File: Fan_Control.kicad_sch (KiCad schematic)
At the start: 7 parts, among them IC1 ADT7470ARQZ-REEL7

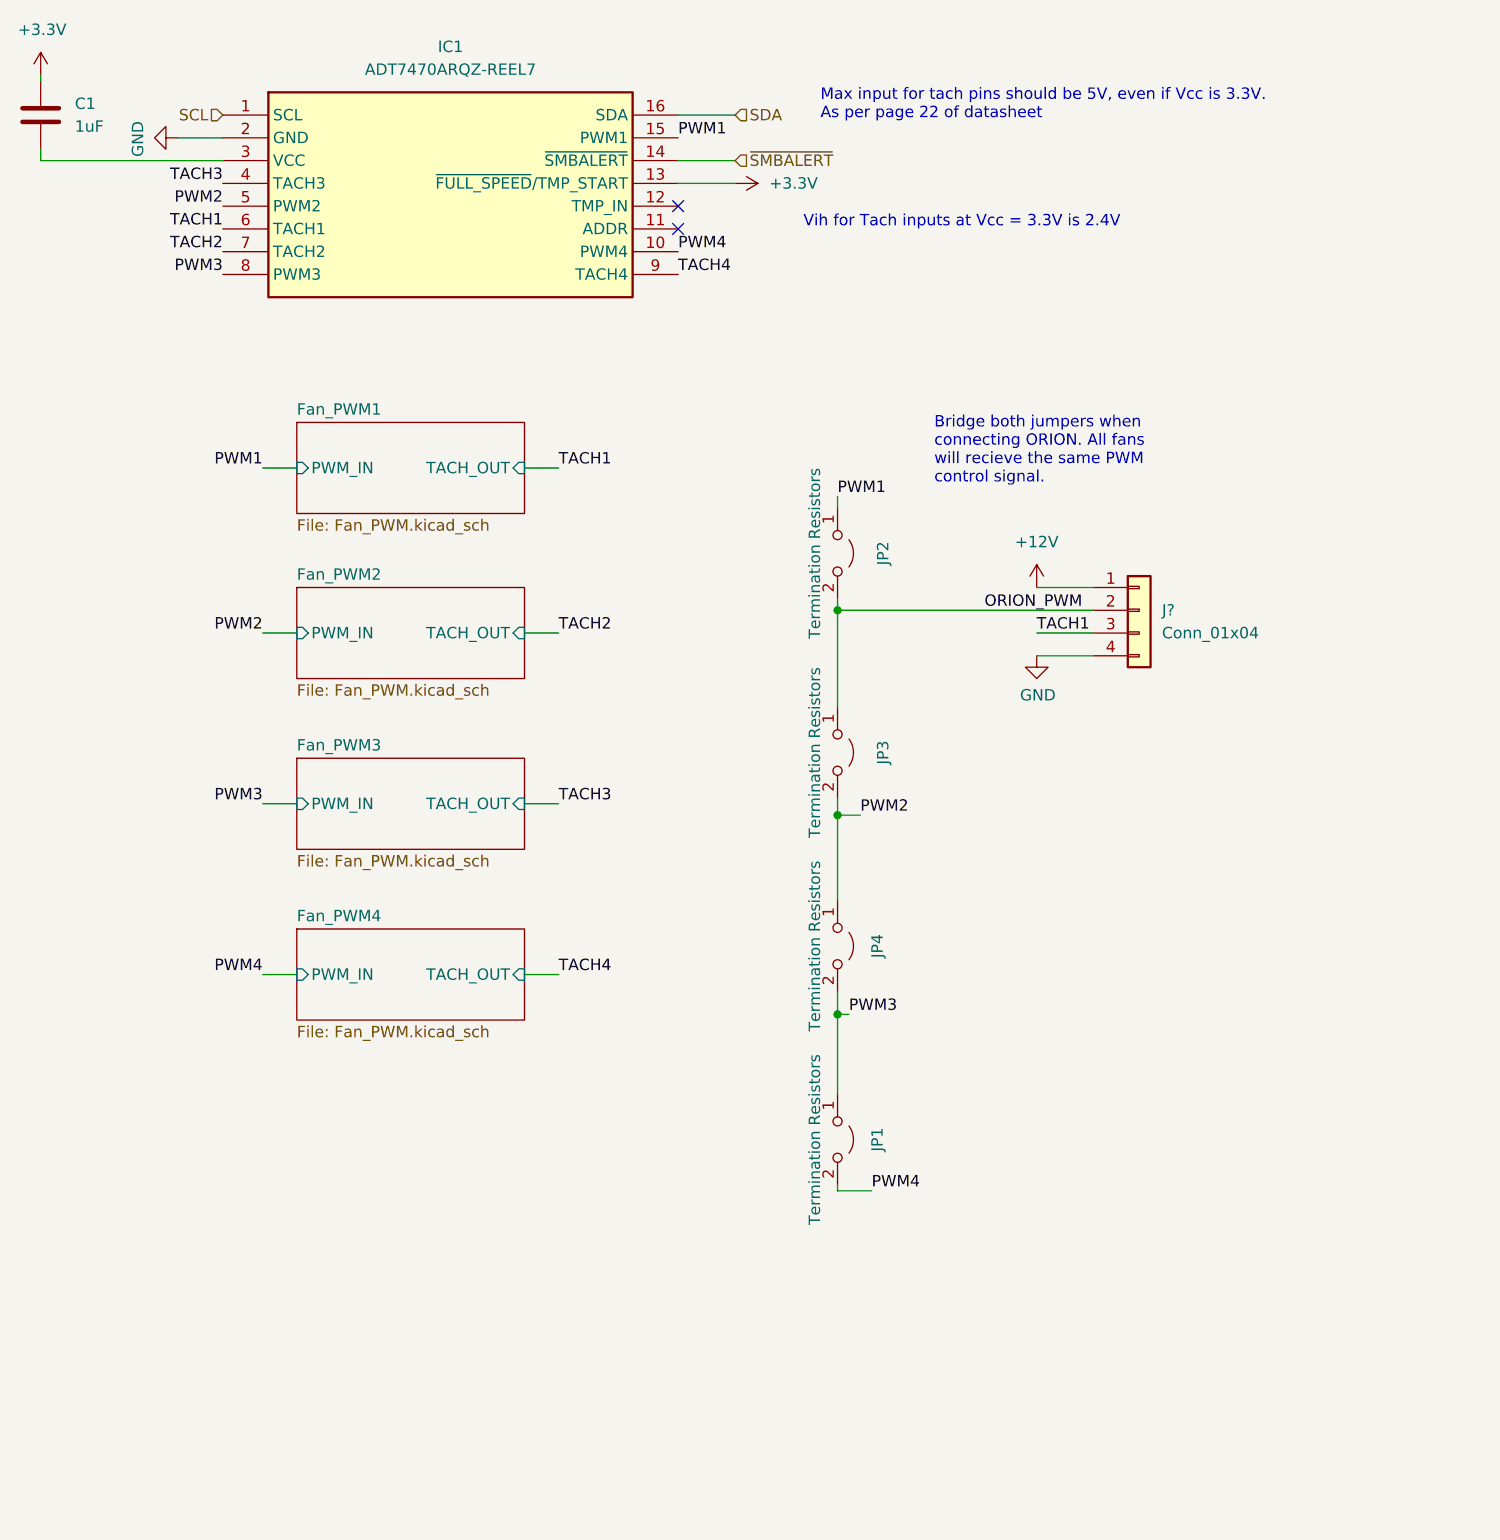
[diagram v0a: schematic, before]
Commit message: why your schematic so broken >:(
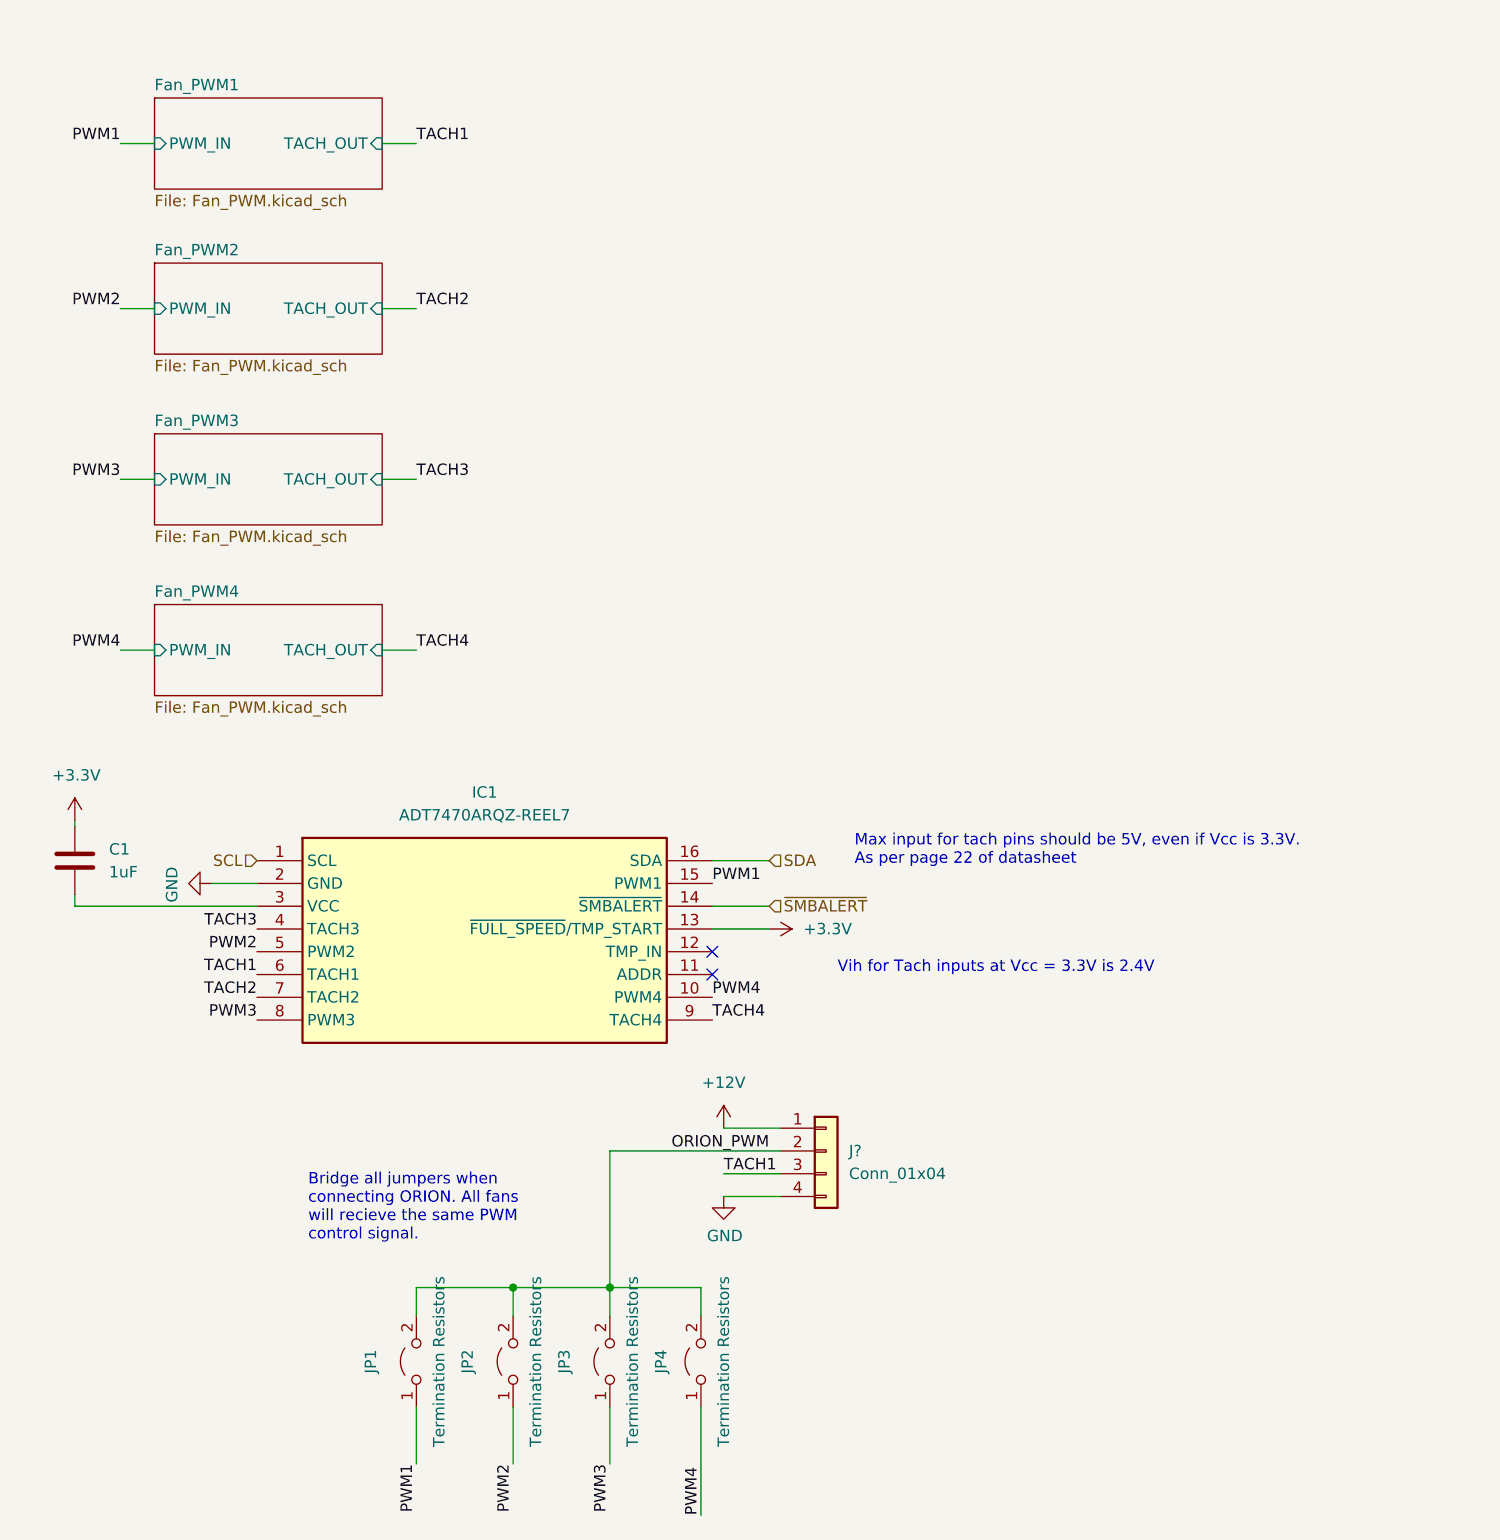
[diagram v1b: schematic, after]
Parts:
- renumbered JP2 to JP1, JP3 to JP2, JP4 to JP3, JP1 to JP4
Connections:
- net ORION_PWM: now also JP2.2 (B), JP3.2 (B), JP4.2 (B); no longer JP2.1 (A)
- net PWM2: now also JP2.1 (A); no longer JP2.2 (B), JP3.1 (A)
- net PWM3: now also JP3.1 (A); no longer JP3.2 (B), JP4.1 (A)
- net PWM4: now also JP4.1 (A); no longer JP4.2 (B)
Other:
- note added: "Bridge all jumpers when connecting ORION. All fans will recieve the same PWM control signal."
- note removed: "Bridge both jumpers when connecting ORION. All fans will recieve the same PWM control signal."
- moved on the sheet: C1, IC1, J?, JP1, JP2, JP3, JP4
